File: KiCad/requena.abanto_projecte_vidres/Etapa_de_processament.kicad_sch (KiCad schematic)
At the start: 45 parts, among them J1 Conn_01x05, J2 Conn_01x04_Socket, J3 DE9_Pins, J4 DE9_Pins, SW1 SW_Push_SPDT, SW2 SW_Push, SW3 SW_Omron_B3FS, SW4 SW_Omron_B3FS, SW5 SW_Omron_B3FS, SW6 SW_Omron_B3FS, U10 NMUX1308PW, U7 PN5120A0HN1, U8 PIC24HJ128GP502, U9 TJA1051TK-3, Y1 27.12 MHz, Y2 8 MHz

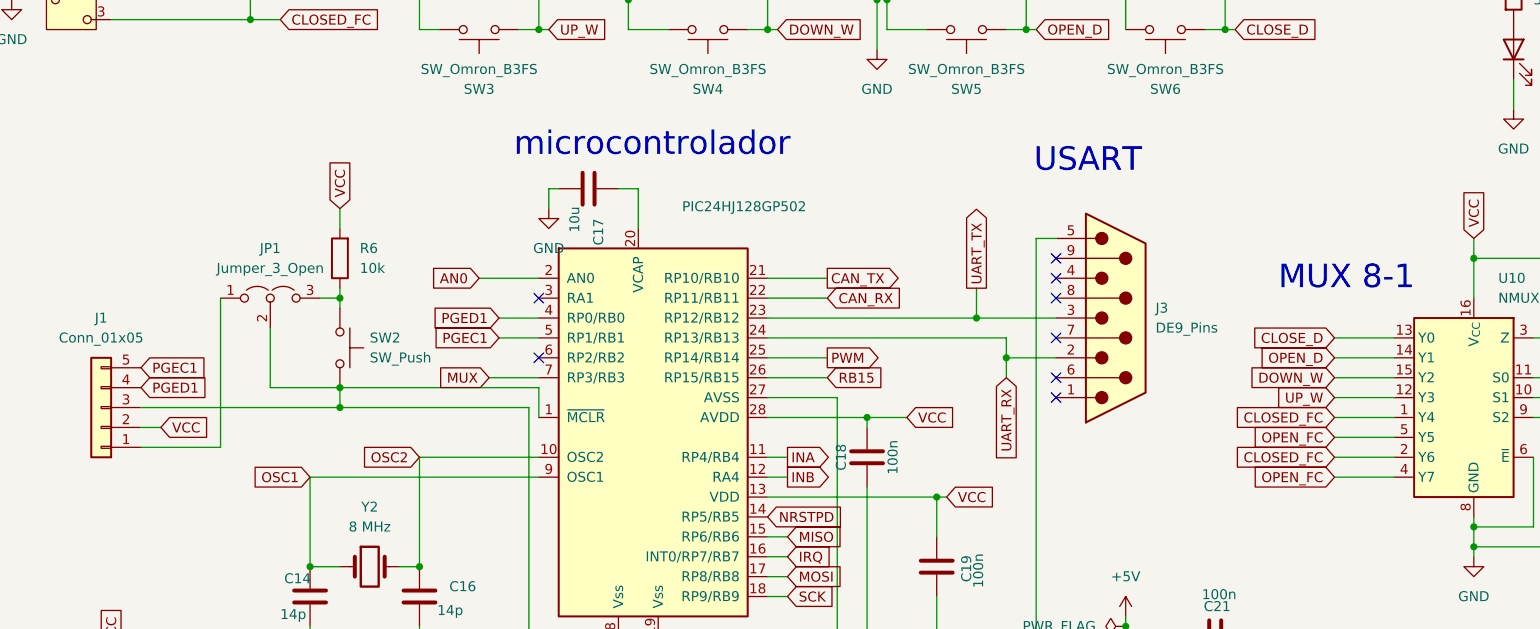
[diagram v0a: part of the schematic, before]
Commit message: milora_esquema_i_layoutcomençat
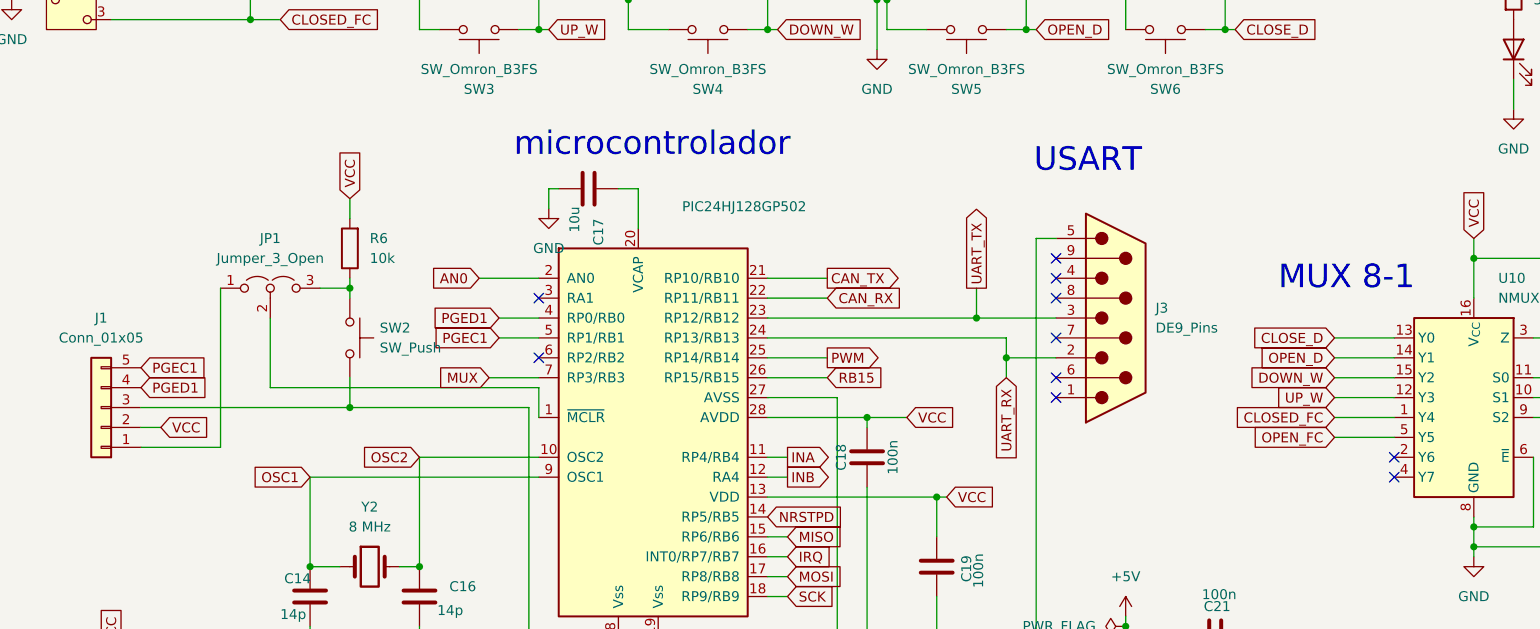
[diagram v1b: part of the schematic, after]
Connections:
- net CLOSED_FC: no longer U10.2 (Y6)
- net GND: no longer JP1.2 (C), U8.1 (~{MCLR})
- net OPEN_FC: no longer U10.4 (Y7)
- new net: JP1.2 (C), U8.1 (~{MCLR})
- no-connect marks 20 -> 22
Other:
- moved on the sheet: JP1, R6, SW2
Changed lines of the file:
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@@
 	)
 	(junction
-		(at 106.68 74.93)
-		(diameter 0)
-		(color 0 0 0 0)
-	)
-	(junction
-		(at 106.68 86.36)
+		(at 107.95 73.66)
 		(diameter 0)
 		(color 0 0 0 0)
@@
 	)
 	(junction
+		(at 107.95 88.9)
+		(diameter 0)
+		(color 0 0 0 0)
+	)
+	(junction
 		(at 83.82 22.86)
 		(diameter 0)
@@
 		(color 0 0 0 0)
 	)
-	(junction
-		(at 106.68 88.9)
-		(diameter 0)
-		(color 0 0 0 0)
+	(no_connect
+		(at 241.3 95.25)
 	)
 	(no_connect
@@
 	)
 	(no_connect
+		(at 241.3 97.79)
+	)
+	(no_connect
 		(at 55.88 170.18)
 	)
@@
 	(wire
 		(pts
-			(xy 104.14 74.93) (xy 106.68 74.93)
-		)
-		(stroke
-			(width 0)
-			(type default)
-		)
-	)
-	(wire
-		(pts
 			(xy 68.58 180.34) (xy 68.58 187.96)
 		)
@@
 	(wire
 		(pts
-			(xy 97.79 78.74) (xy 97.79 86.36)
+			(xy 97.79 77.47) (xy 97.79 86.36)
 		)
 		(stroke
@@
 	(wire
 		(pts
-			(xy 97.79 86.36) (xy 106.68 86.36)
+			(xy 97.79 86.36) (xy 132.08 86.36)
 		)
 		(stroke
@@
 	(wire
 		(pts
+			(xy 104.14 73.66) (xy 107.95 73.66)
+		)
+		(stroke
+			(width 0)
+			(type default)
+		)
+	)
+	(wire
+		(pts
 			(xy 176.53 36.83) (xy 207.01 36.83)
 		)
@@
 	(wire
 		(pts
-			(xy 106.68 73.66) (xy 106.68 74.93)
+			(xy 107.95 72.39) (xy 107.95 73.66)
 		)
 		(stroke
@@
 	(wire
 		(pts
-			(xy 130.81 88.9) (xy 106.68 88.9)
-		)
-		(stroke
-			(width 0)
-			(type default)
-		)
-	)
-	(wire
-		(pts
 			(xy 76.2 180.34) (xy 76.2 187.96)
 		)
@@
 	(wire
 		(pts
+			(xy 107.95 85.09) (xy 107.95 88.9)
+		)
+		(stroke
+			(width 0)
+			(type default)
+		)
+	)
+	(wire
+		(pts
 			(xy 95.25 39.37) (xy 99.06 39.37)
 		)
@@
 	(wire
 		(pts
-			(xy 106.68 74.93) (xy 106.68 76.2)
+			(xy 107.95 73.66) (xy 107.95 74.93)
 		)
 		(stroke
@@
 	(wire
 		(pts
-			(xy 91.44 74.93) (xy 91.44 93.98)
-		)
-		(stroke
-			(width 0)
-			(type default)
-		)
-	)
-	(wire
-		(pts
-			(xy 233.68 95.25) (xy 241.3 95.25)
+			(xy 91.44 73.66) (xy 91.44 93.98)
 		)
 		(stroke
@@
 	(wire
 		(pts
-			(xy 233.68 97.79) (xy 241.3 97.79)
-		)
-		(stroke
-			(width 0)
-			(type default)
-		)
-	)
-	(wire
-		(pts
 			(xy 144.78 120.65) (xy 142.24 120.65)
 		)
@@
 	(wire
 		(pts
-			(xy 106.68 86.36) (xy 106.68 88.9)
-		)
-		(stroke
-			(width 0)
-			(type default)
-		)
-	)
-	(wire
-		(pts
 			(xy 91.44 157.48) (xy 96.52 157.48)
 		)
@@
 	(wire
 		(pts
-			(xy 106.68 86.36) (xy 132.08 86.36)
-		)
-		(stroke
-			(width 0)
-			(type default)
-		)
-	)
-	(wire
-		(pts
 			(xy 24.13 128.27) (xy 34.29 128.27)
 		)
@@
 	(wire
 		(pts
-			(xy 106.68 63.5) (xy 106.68 66.04)
+			(xy 107.95 62.23) (xy 107.95 64.77)
 		)
 		(stroke
@@
 	(wire
 		(pts
+			(xy 107.95 88.9) (xy 130.81 88.9)
+		)
+		(stroke
+			(width 0)
+			(type default)
+		)
+	)
+	(wire
+		(pts
 			(xy 194.31 40.64) (xy 194.31 35.56)
 		)
@@
 	(wire
 		(pts
-			(xy 81.28 88.9) (xy 106.68 88.9)
+			(xy 81.28 88.9) (xy 107.95 88.9)
 		)
 		(stroke
@@
 	(global_label "VCC"
 		(shape input)
-		(at 106.68 63.5 90)
+		(at 107.95 62.23 90)
 		(fields_autoplaced yes)
 		(effects
@@
 		)
 		(property "Intersheetrefs" "${INTERSHEET_REFS}"
-			(at 106.68 56.8862 90)
+			(at 107.95 55.6162 90)
 			(effects
 				(font
@@
 		)
 	)
-	(global_label "OPEN_FC"
-		(shape input)
-		(at 233.68 97.79 180)
-		(fields_autoplaced yes)
-		(effects
-			(font
-				(size 1.27 1.27)
-			)
-			(justify right)
-		)
-		(property "Intersheetrefs" "${INTERSHEET_REFS}"
-			(at 222.2886 97.79 0)
-			(effects
-				(font
-					(size 1.27 1.27)
-				)
-				(justify right)
-				(hide yes)
-			)
-		)
-	)
 	(global_label "VCC"
 		(shape input)
@@
 		)
 	)
-	(global_label "CLOSED_FC"
-		(shape input)
-		(at 233.68 95.25 180)
-		(fields_autoplaced yes)
-		(effects
-			(font
-				(size 1.27 1.27)
-			)
-			(justify right)
-		)
-		(property "Intersheetrefs" "${INTERSHEET_REFS}"
-			(at 220.1115 95.25 0)
-			(effects
-				(font
-					(size 1.27 1.27)
-				)
-				(justify right)
-				(hide yes)
-			)
-		)
-	)
 	(symbol
 		(lib_id "Interface_CAN_LIN:TJA1051TK-3")
@@
 	(symbol
 		(lib_id "Switch:SW_Push")
-		(at 106.68 81.28 270)
+		(at 107.95 80.01 270)
 		(unit 1)
 		(exclude_from_sim no)
@@
 		(fields_autoplaced yes)
 		(property "Reference" "SW2"
-			(at 110.49 80.0099 90)
+			(at 111.76 78.7399 90)
 			(effects
 				(font
@@
 		)
 		(property "Value" "SW_Push"
-			(at 110.49 82.5499 90)
+			(at 111.76 81.2799 90)
 			(effects
 				(font
@@
 		)
 		(property "Footprint" "Button_Switch_SMD:SW_Push_1P1T_NO_E-Switch_TL3301NxxxxxG"
-			(at 111.76 81.28 0)
+			(at 113.03 80.01 0)
 			(effects
 				(font
@@
 		)
 		(property "Datasheet" "~"
-			(at 111.76 81.28 0)
+			(at 113.03 80.01 0)
 			(effects
 				(font
@@
 		)
 		(property "Description" "Push button switch, generic, two pins"
-			(at 106.68 81.28 0)
+			(at 107.95 80.01 0)
 			(effects
 				(font
@@
 	(symbol
 		(lib_id "Device:R")
-		(at 106.68 69.85 180)
+		(at 107.95 68.58 180)
 		(unit 1)
 		(exclude_from_sim no)
@@
 		(fields_autoplaced yes)
 		(property "Reference" "R6"
-			(at 109.22 68.5799 0)
+			(at 110.49 67.3099 0)
 			(effects
 				(font
@@
 		)
 		(property "Value" "10k"
-			(at 109.22 71.1199 0)
+			(at 110.49 69.8499 0)
 			(effects
 				(font
@@
 		)
 		(property "Footprint" "Resistor_SMD:R_1206_3216Metric"
-			(at 108.458 69.85 90)
+			(at 109.728 68.58 90)
 			(effects
 				(font
@@
 		)
 		(property "Datasheet" "~"
-			(at 106.68 69.85 0)
+			(at 107.95 68.58 0)
 			(effects
 				(font
@@
 		)
 		(property "Description" "Resistor"
-			(at 106.68 69.85 0)
+			(at 107.95 68.58 0)
 			(effects
 				(font
@@
 	(symbol
 		(lib_id "Jumper:Jumper_3_Open")
-		(at 97.79 74.93 0)
+		(at 97.79 73.66 0)
 		(unit 1)
 		(exclude_from_sim no)
@@
 		(fields_autoplaced yes)
 		(property "Reference" "JP1"
-			(at 97.79 68.58 0)
+			(at 97.79 67.31 0)
 			(effects
 				(font
@@
 		)
 		(property "Value" "Jumper_3_Open"
-			(at 97.79 71.12 0)
+			(at 97.79 69.85 0)
 			(effects
 				(font
@@
 		)
 		(property "Footprint" "Connector_PinHeader_2.54mm:PinHeader_1x03_P2.54mm_Horizontal"
-			(at 97.79 74.93 0)
+			(at 97.79 73.66 0)
 			(effects
 				(font
@@
 		)
 		(property "Datasheet" "~"
-			(at 97.79 74.93 0)
+			(at 97.79 73.66 0)
 			(effects
 				(font
@@
 		)
 		(property "Description" "Jumper, 3-pole, both open"
-			(at 97.79 74.93 0)
+			(at 97.79 73.66 0)
 			(effects
 				(font
